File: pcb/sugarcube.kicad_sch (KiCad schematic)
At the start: 0 parts

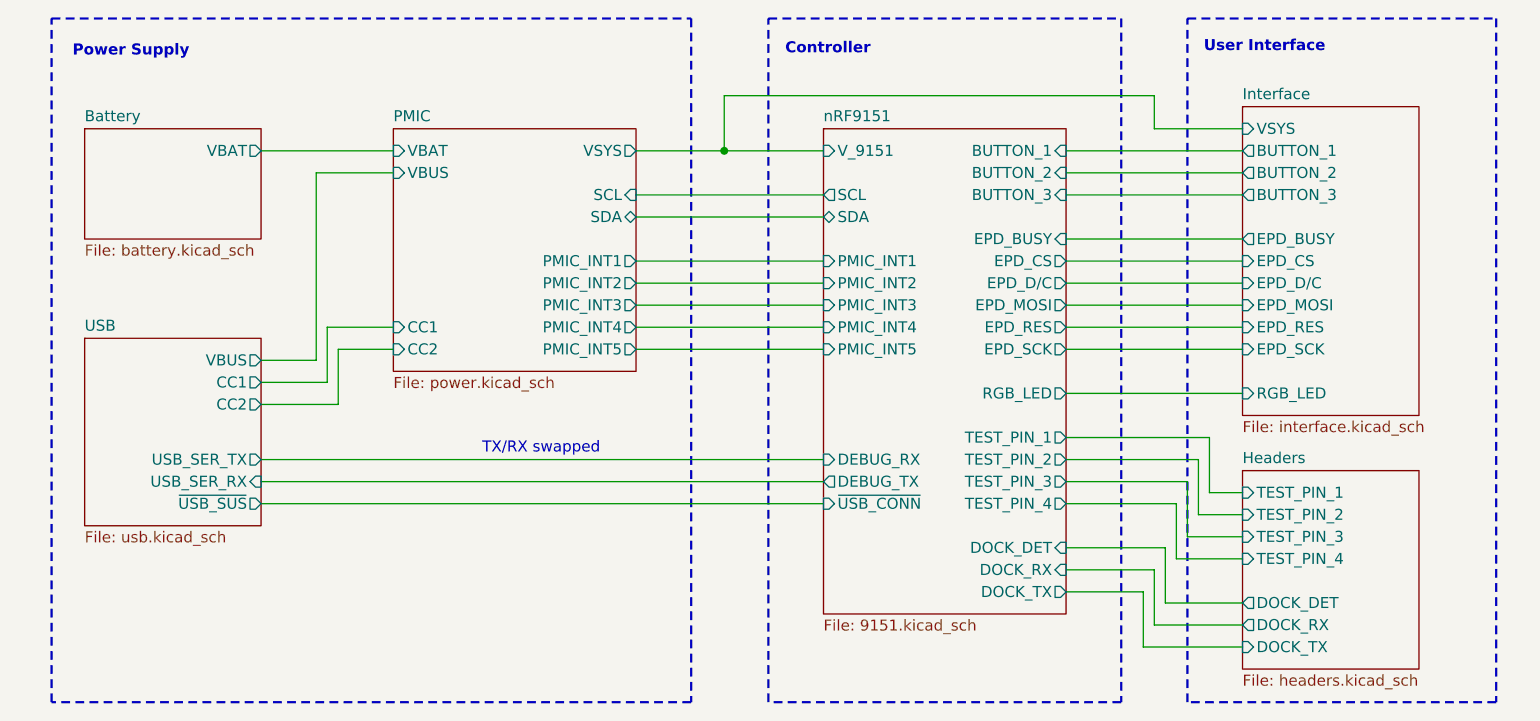
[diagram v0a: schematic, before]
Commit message: clean up
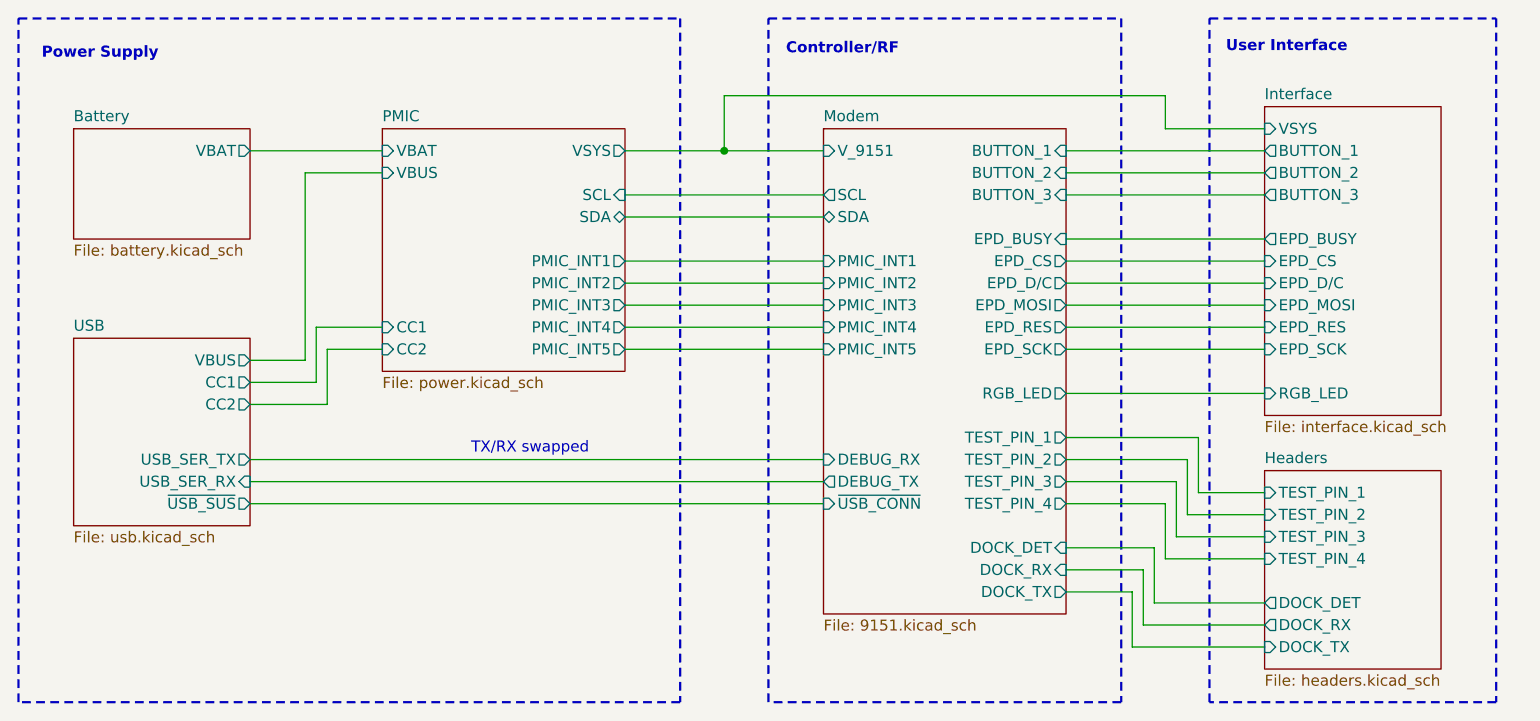
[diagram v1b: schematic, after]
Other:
- sheet nRF9151 renamed Modem
- note added: "Controller/RF"
- note removed: "Controller"
